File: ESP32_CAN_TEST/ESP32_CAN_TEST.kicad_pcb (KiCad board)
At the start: 2 copper layers, 45.7 x 45.7 mm, 25 parts, among them J1 5V in, J2 Conn_01x05, J3 Molex_2x2, J4 Conn_01x05, J5 i2C, J6 UART, SW1 EN, SW2 EN, U1 AMS1117, U2 ESP32-WROOM-32, U3 SN65HVD230

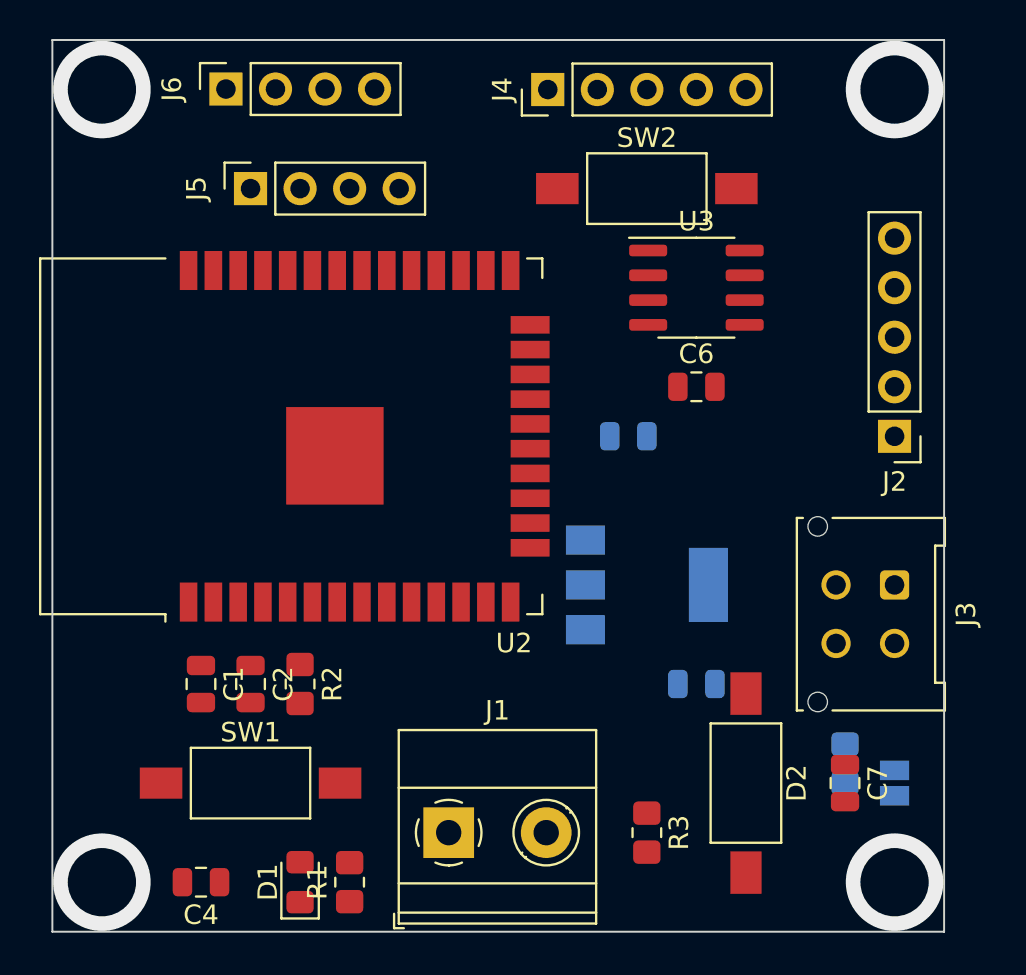
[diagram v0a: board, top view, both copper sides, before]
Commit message: update
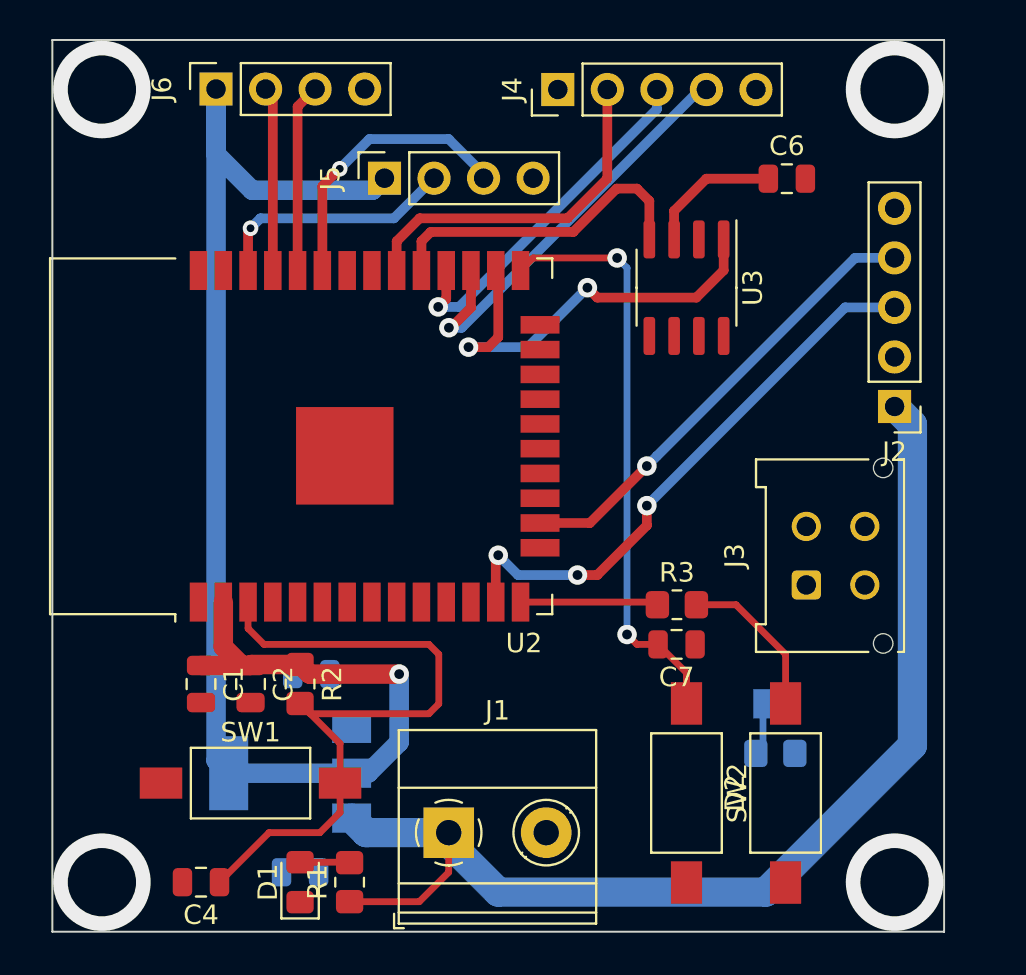
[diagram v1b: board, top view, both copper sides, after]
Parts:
- moved SW2 31.1 mm to (134.1, 79.2), turned to -90 degrees
- moved C3 28.0 mm to (114.3, 83.3), turned to 180 degrees
- moved U1 20.7 mm to (113.8, 78.2), turned to 180 degrees
- moved C5 19.8 mm to (114.9, 73.2), turned to 0 degrees
- moved R3 11.8 mm to (133.6, 69.6), turned to 0 degrees
- moved C6 11.6 mm to (139.3, 47.8)
- moved C7 11.2 mm to (133.6, 71.6), turned to 180 degrees
- moved JP1 7.33 mm to (138.7, 74.7), turned to 180 degrees
- moved J5 6.89 mm to (118.6, 47.7)
- moved J3 4.52 mm to (140.3, 68.6), turned to 90 degrees
- moved R4 3.61 mm to (138.7, 77.2), turned to 0 degrees
- moved D2 2.09 mm to (139.2, 79.2), turned to 90 degrees
- moved J2 1.53 mm to (144.8, 59.4)
- moved J4 0.51 mm to (127.5, 43.2)
- moved U3 0.51 mm to (134.1, 53.3), turned to -90 degrees
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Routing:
- net +3V3: track 0.00 -> 82.2 mm, vias 0 -> 1
- net +5V: track 0.00 -> 59.2 mm
- net Net-(C4-Pad1): track 0.00 -> 35.9 mm
- net Net-(C7-Pad2): track 0.00 -> 30.2 mm, vias 0 -> 2
- net /IO14: track 0.00 -> 29.5 mm, vias 0 -> 3
- net /IO13: track 0.00 -> 23.8 mm, vias 0 -> 1
- net /CAN_TX: track 0.00 -> 21.9 mm, vias 0 -> 2
- net /IO16: track 0.00 -> 21.7 mm, vias 0 -> 1
- net /IO17: track 0.00 -> 18.5 mm, vias 0 -> 1
- net /IO18: track 0.00 -> 18.2 mm
- net /CAN_RX: track 0.00 -> 16.5 mm
- net /SDA: track 0.00 -> 14.6 mm, vias 0 -> 1
- net /SCL: track 0.00 -> 12.7 mm, vias 0 -> 1
- net /RXD: track 0.00 -> 9.68 mm
- net /TXD: track 0.00 -> 9.46 mm
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
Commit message: update
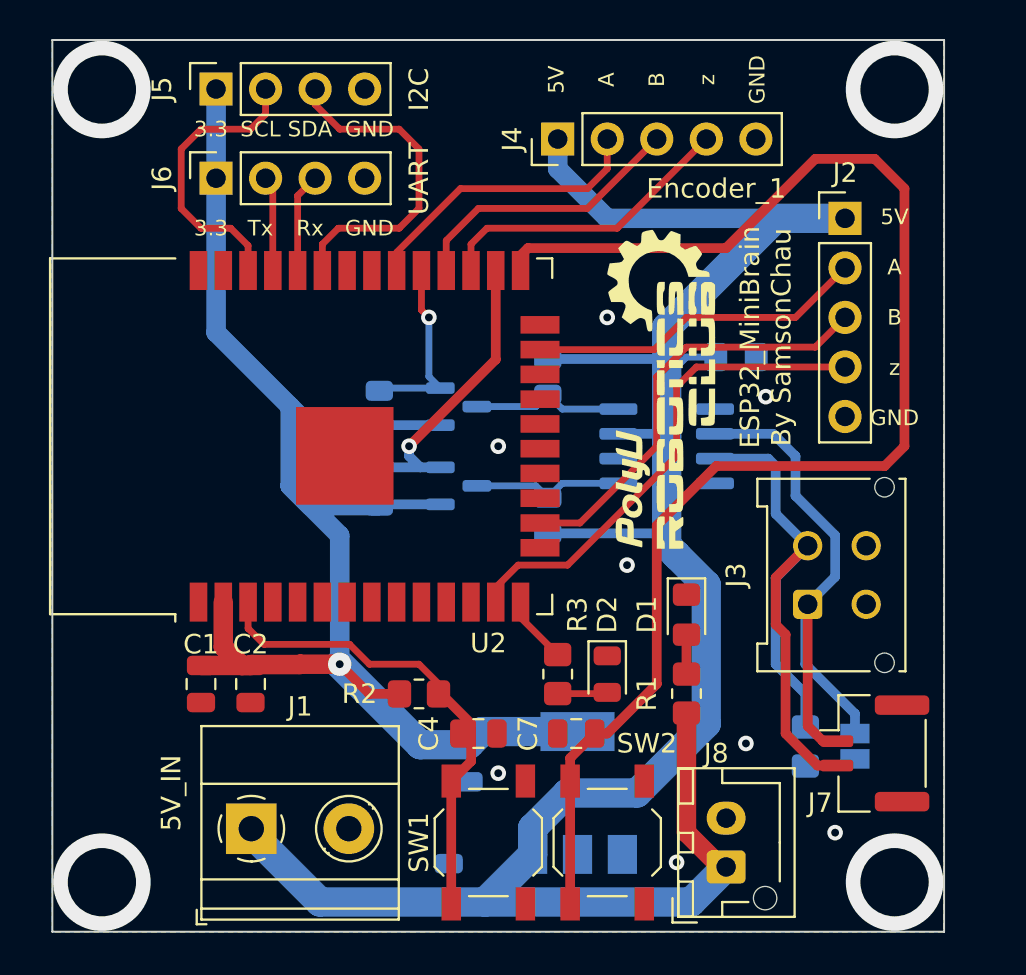
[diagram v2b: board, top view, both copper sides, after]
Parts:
- added G***: LOGO, PolyuRobotics:Club_logo, F.Cu at (133.1, 58.4)
- added J7: GH1.25, Connector_JST:JST_GH_BM02B-GHS-TBT_1x02-1MP_P1.25mm_Vertical, F.Cu at (143.8, 77.2)
- added J8: JST_2.54, Connector_JST:JST_XH_B2B-XH-AM_1x02_P2.50mm_Vertical, F.Cu at (136.1, 83.0)
- added Q1: 2N7002, Package_TO_SOT_SMD:SOT-23, B.Cu at (122.4, 63.5)
- added Q2: 2N7002, Package_TO_SOT_SMD:SOT-23, B.Cu at (122.4, 59.4)
- added R5: 10K, Resistor_SMD:R_0805_2012Metric, B.Cu at (118.4, 63.6)
- added R6: 10K, Resistor_SMD:R_0805_2012Metric, B.Cu at (118.4, 59.5)
- added R7: 10K, Resistor_SMD:R_0805_2012Metric, B.Cu at (127.0, 65.0)
- added R8: 10K, Resistor_SMD:R_0805_2012Metric, B.Cu at (127.0, 57.9)
- C6: value 0.1uf -> 100nF; footprint Capacitor_SMD:C_0805_2012Metric -> Capacitor_SMD:C_0805_2012Metric_Pad1.18x1.45mm_HandSolder; moved to B.Cu
- D2: footprint Button_Switch_SMD:SW_SPST_FSMSM -> LED_SMD:LED_0805_2012Metric
- J2: value Conn_01x05 -> Encoder_1
- J4: value Conn_01x05 -> Encoder2
- SW1, SW2: footprint Button_Switch_SMD:SW_SPST_FSMSM -> Button_Switch_SMD:SW_SPST_TL3342
- U3: value SN65HVD230 -> TJA1050; moved to B.Cu
- moved D1 24.1 mm to (134.1, 70.1), turned to -90 degrees
- moved R1 19.8 mm to (134.1, 74.2)
- moved C4 16.1 mm to (123.4, 76.2), turned to 0 degrees
- moved U1 14.8 mm to (128.5, 79.2), turned to 90 degrees
- moved SW1 12.6 mm to (124.0, 81.8), turned to -90 degrees
- moved D2 11.0 mm to (130.0, 73.2), turned to -90 degrees
- moved J1 10.1 mm to (111.8, 81.1)
- moved J2 9.98 mm to (142.2, 49.8), turned to 0 degrees
- moved J5 9.77 mm to (110.0, 43.2)
- moved C6 9.51 mm to (136.7, 56.9)
- moved C5 9.27 mm to (122.9, 77.7), turned to -90 degrees
- moved U3 8.19 mm to (133.1, 61.5), turned to 0 degrees
- moved C3 7.64 mm to (121.9, 83.8), turned to 90 degrees
- moved R3 7.07 mm to (127.5, 73.2), turned to -90 degrees
- moved C7 6.88 mm to (128.5, 76.2), turned to 0 degrees
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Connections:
- C6 pad 1: +3V3 -> +5V
- J2 pad 3: /IO14 -> /IO13
- J2 pad 4: /IO13 -> /IO14
- U3 pad 1: /CAN_TX -> Net-(Q1-Pad3)
- U3 pad 3: +3V3 -> +5V
- U3 pad 4: /CAN_RX -> Net-(Q2-Pad3)
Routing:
- net +5V: track 59.2 -> 118.2 mm
- net Net-(C7-Pad2): track 30.2 -> 72.4 mm, vias 2 -> 0
- net /CANL-: track 0.00 -> 32.5 mm
- net /CANH+: track 0.00 -> 29.4 mm
- net /IO15: track 0.00 -> 17.4 mm
- net Net-(C4-Pad1): track 35.9 -> 24.8 mm
- net Net-(Q1-Pad3): track 0.00 -> 7.81 mm
- net Net-(Q2-Pad3): track 0.00 -> 7.81 mm
- net /CAN_RX: track 16.5 -> 9.61 mm, vias 0 -> 1
- net /CAN_TX: track 21.9 -> 15.4 mm, vias 2 -> 1
- net /IO16: track 21.7 -> 15.6 mm, vias 1 -> 0
- net Net-(D2-Pad2): track 8.15 -> 2.57 mm
- net +3V3: track 82.2 -> 77.1 mm
- net /TXD: track 9.46 -> 4.89 mm
- net /RXD: track 9.68 -> 5.11 mm
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- added copper zone on B.Cu, net GND
- added copper zone on F.Cu, net GND
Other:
- board text added: "3.3"
- board text added: "5V"
- board text added: "5V A B z GND"
- board text added: "5V_IN"
- board text added: "ESP32_MiniBrain By SamsonChau"
- board text added: "Encoder_1"
- board text added: "GND"
- board text added: "I2C"
- board text added: "Rx"
- board text added: "SCL"
- board text added: "SDA"
- board text added: "Tx"
- board text added: "UART"
